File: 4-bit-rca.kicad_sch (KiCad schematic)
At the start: 27 parts, among them J1 CIN & COUT, SW1 SW_DIP_x08, U1 74HC86, U2 74HC08, U3 74HC32, U4 74HC08, U5 74HC86, U6 L7805

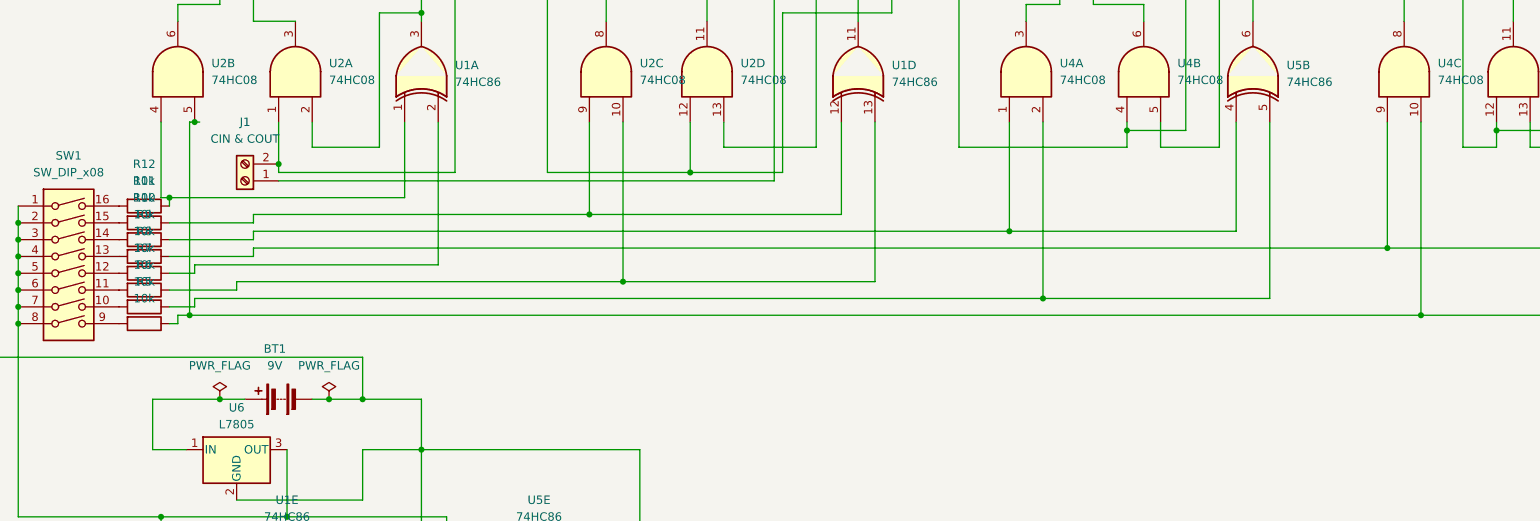
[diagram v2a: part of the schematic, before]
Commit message: a
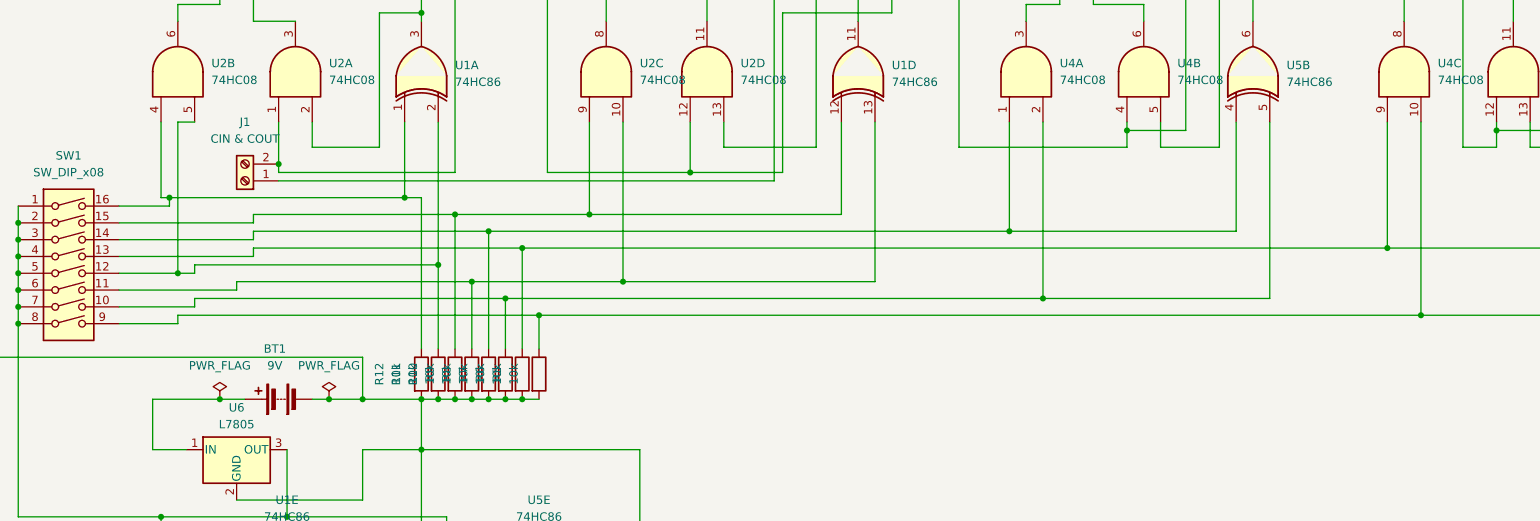
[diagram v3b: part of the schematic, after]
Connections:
- net at BT1.2 (-), D1.1 (K), D2.1 (K)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: now also R10.2, R11.2, R12.2, R5.2, R6.2, R7.2, R8.2, R9.2
- net at U1.13, U2.10: now also R9.1, SW1.11; no longer R7.1
- net at SW1.10: now also R7.1, U4.2, U5.5; no longer R6.2
- net at SW1.12: now also R11.1, U1.2, U2.5; no longer R8.2
- net at SW1.13: now also R6.1, U4.9, U5.9; no longer R9.2
- net at SW1.14: now also R8.1, U4.1, U5.4; no longer R10.2
- net at SW1.15: now also R10.1, U1.12, U2.9; no longer R11.2
- net at SW1.16: now also R12.1, U1.1, U2.4; no longer R12.2
- net at SW1.9: now also R5.1, U4.10, U5.10; no longer R5.2
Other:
- moved on the sheet: R10, R11, R12, R5, R6, R7, R8, R9
